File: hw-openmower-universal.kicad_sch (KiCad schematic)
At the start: 32 parts

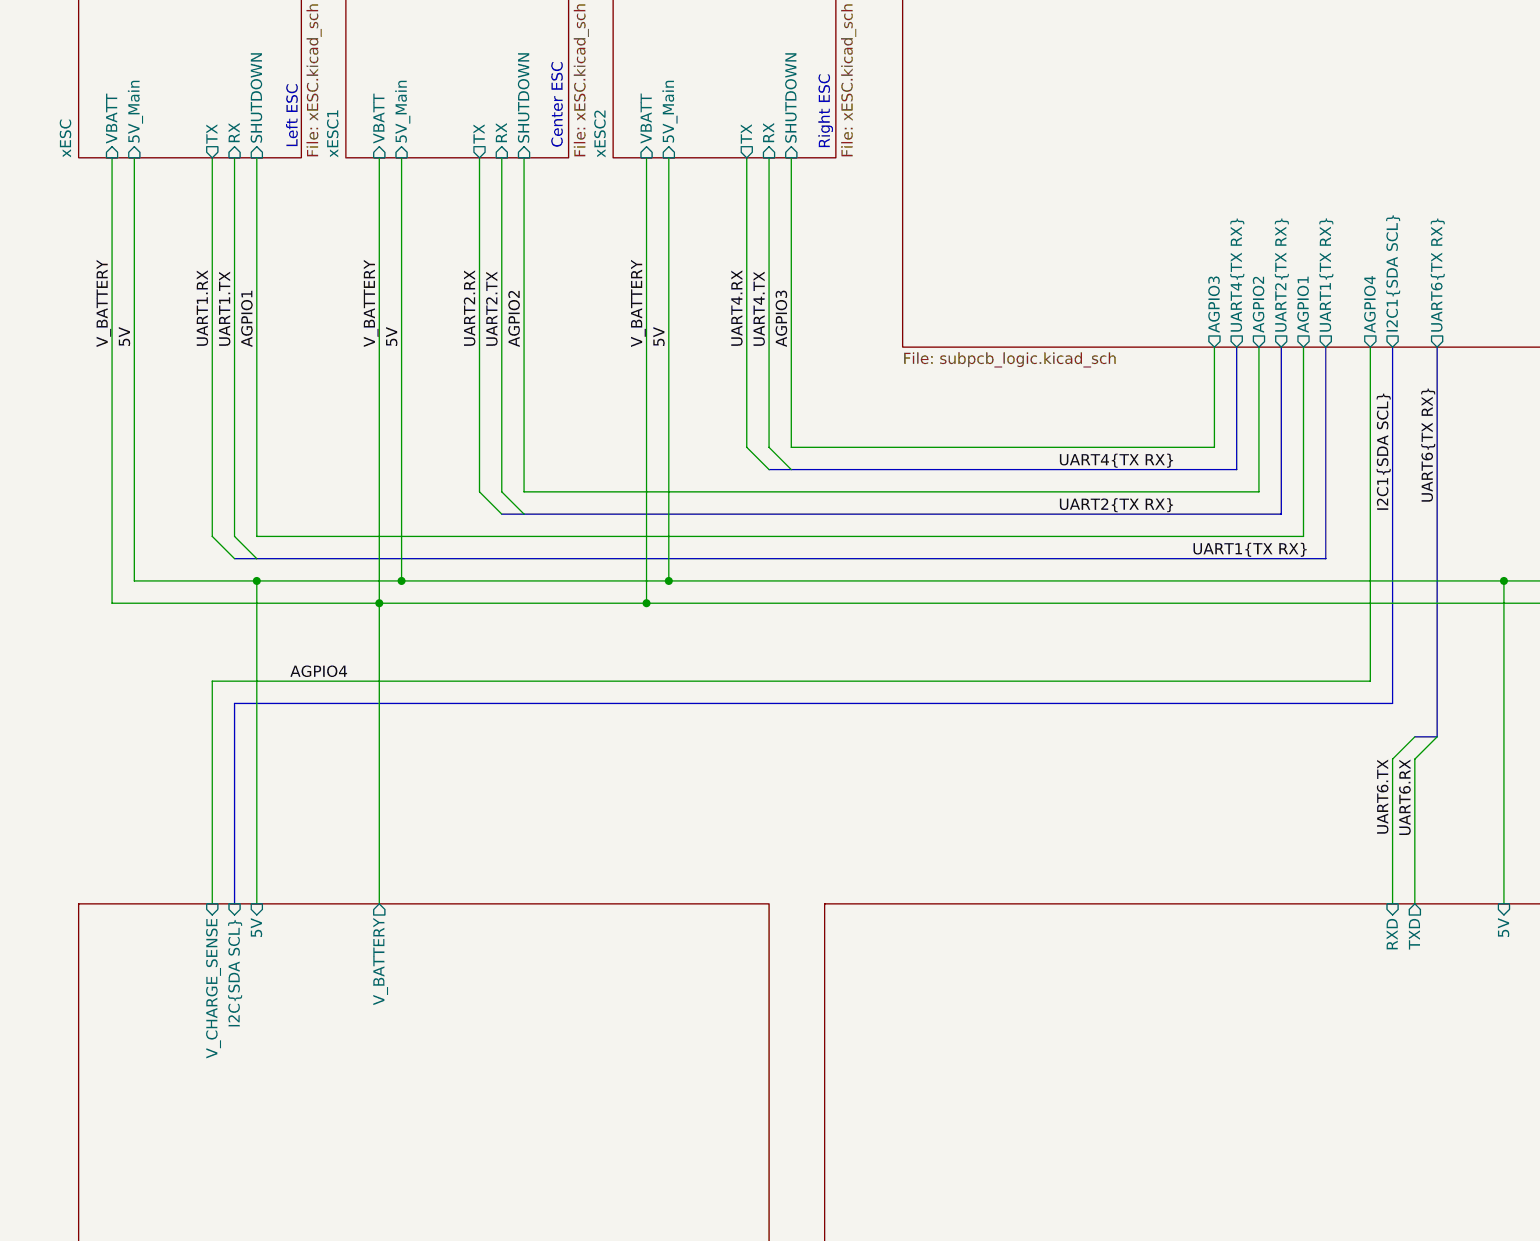
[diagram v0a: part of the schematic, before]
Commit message: wip
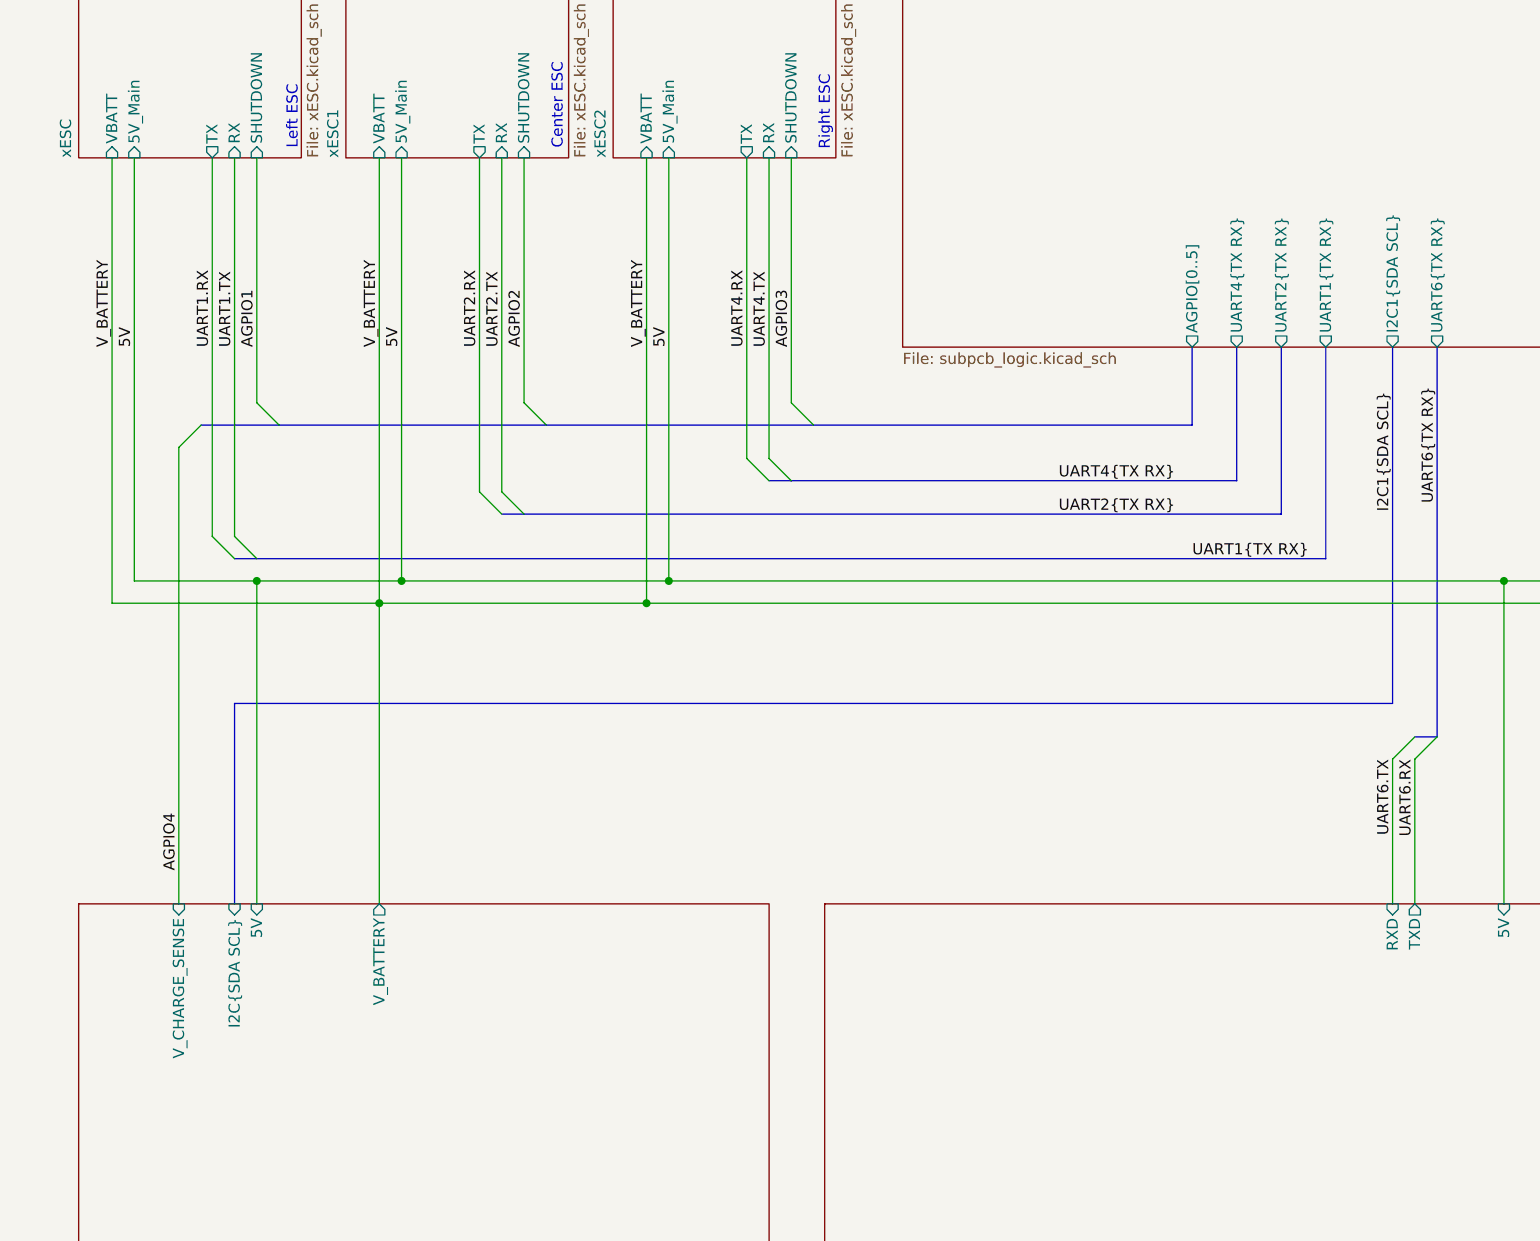
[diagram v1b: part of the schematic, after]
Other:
- sheet subpcb_logic ports: added AGPIO[0..5]; removed AGPIO1, AGPIO2, AGPIO3, AGPIO4
